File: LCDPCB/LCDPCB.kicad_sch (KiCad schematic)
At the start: 32 parts, among them J1 Sockets, J2 Hot Plug, J3 Programming Header, J4 Conn_01x08_Male, J5 Conn_01x08_Male, SW1 SW_Push, U1 STM32F091RCT6, U2 LD1117S12TR_SOT223

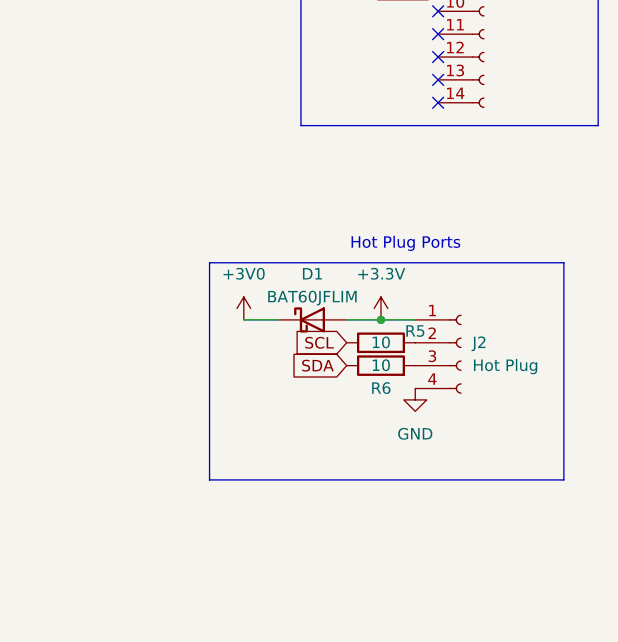
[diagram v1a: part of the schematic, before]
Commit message: edits
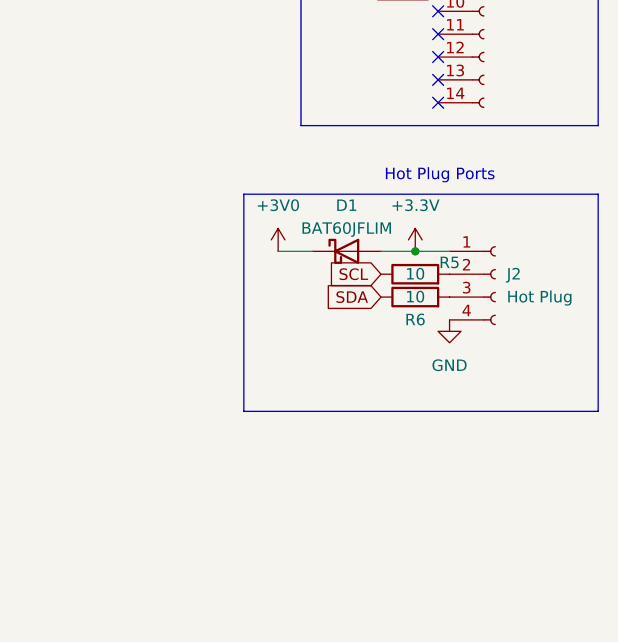
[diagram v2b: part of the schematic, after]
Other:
- moved on the sheet: D1, J2, R5, R6

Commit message: submodule casing files
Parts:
- C2: footprint lib_file:10uF -> lib_file:new10uf
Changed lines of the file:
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@@
       (effects (font (size 1.27 1.27)) (justify left))
     )
-    (property "Footprint" "lib_file:10uF" (id 2) (at 27.6352 82.55 0)
+    (property "Footprint" "lib_file:new10uf" (id 2) (at 27.6352 82.55 0)
       (effects (font (size 1.27 1.27)) hide)
     )
@@
     )
     (path "/f24fd606-4838-4530-b0e3-89032e781ead"
-      (reference "C2") (unit 1) (value "10uF") (footprint "lib_file:10uF")
+      (reference "C2") (unit 1) (value "10uF") (footprint "lib_file:new10uf")
     )
     (path "/5da5ad4e-2433-4ba1-8c71-f4c200e15d6f"
